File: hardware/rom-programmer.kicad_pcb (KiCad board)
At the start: 2 copper layers, 100 x 68 mm, 21 parts, among them U1 74HC595, U2 74HC595, U3 28C256

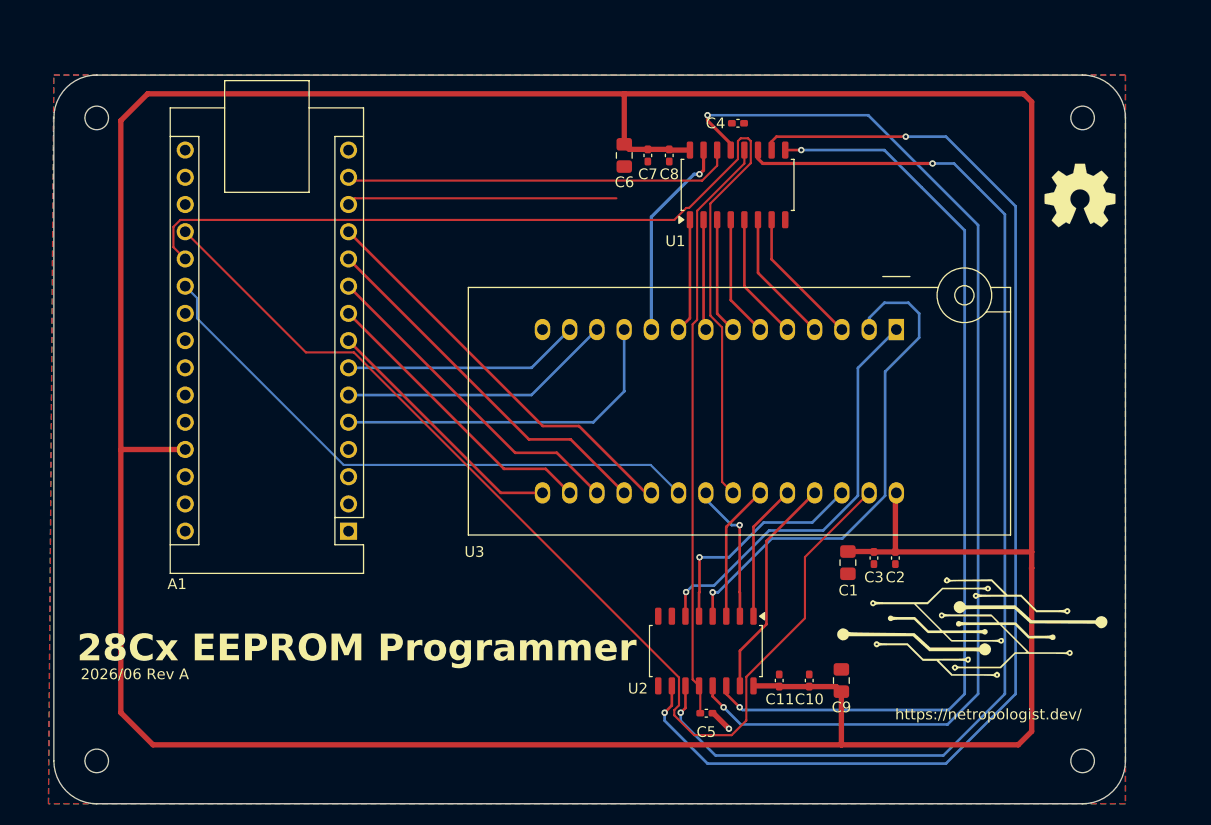
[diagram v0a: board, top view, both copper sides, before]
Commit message: Writing files works
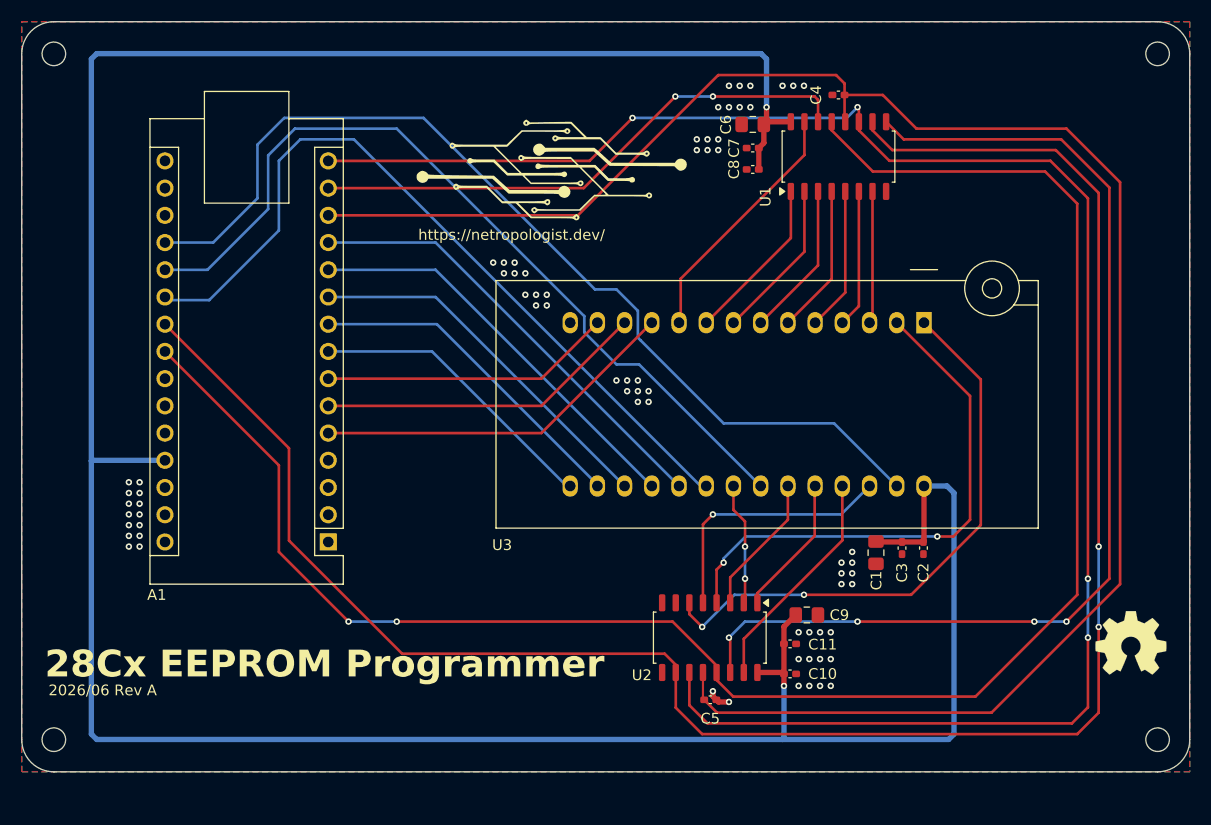
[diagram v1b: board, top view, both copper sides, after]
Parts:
- moved G*** 58.0 mm to (136.5, 71.3)
- moved REF** 42.0 mm to (190.5, 115.5)
- moved C6 12.3 mm to (155.2, 67.1), turned to 180 degrees
- moved C7 9.81 mm to (155.2, 69.3), turned to 180 degrees
- moved U1 9.78 mm to (163.2, 70.1)
- moved C4 9.75 mm to (163.2, 64.4)
- moved H2 9.21 mm to (193.0, 60.5)
- moved C8 7.90 mm to (155.2, 71.3), turned to 180 degrees
- moved H3 7.27 mm to (193.0, 124.5)
- moved H1 7.19 mm to (90.0, 60.5)
- moved C9 6.91 mm to (160.3, 112.9), turned to 0 degrees
- moved H4 4.46 mm to (90.0, 124.5)
- moved C11 3.56 mm to (158.7, 115.6), turned to 0 degrees
- moved C1 2.78 mm to (166.7, 107.1)
- moved C2 2.78 mm to (171.2, 106.6)
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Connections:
- U1 pad 10: /CRCLR -> /~{SRCLR}
- U1 pad 13: /~{SER_OE} -> /~{SEROE}
- U2 pad 10: /CRCLR -> /~{SRCLR}
- U2 pad 13: /~{SER_OE} -> /~{SEROE}
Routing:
- net /~{SRCLR}: track 0.00 -> 184.0 mm, vias 0 -> 2
- net /~{SEROE}: track 0.00 -> 171.0 mm, vias 0 -> 2
- net /CRCLR: track 112.6 -> 0.00 mm, vias 2 -> 0
- net /~{SER_OE}: track 105.4 -> 0.00 mm, vias 2 -> 0
- net /RCLK: track 80.1 -> 171.2 mm
- net +5V: track 340.4 -> 276.7 mm, vias 0 -> 2
- net /SRCLK: track 108.2 -> 166.8 mm, vias 2 -> 4
- net /~{ROM_CE}: track 55.1 -> 74.0 mm
- net /~{ROM_OE}: track 97.1 -> 78.7 mm
- net /SRDATA: track 36.6 -> 51.4 mm, vias 0 -> 2
- net /A14: track 39.0 -> 53.8 mm, vias 1 -> 2
- net /SERO: track 87.3 -> 101.0 mm, vias 2 -> 4
- net /~{ROM_WE}: track 101.1 -> 91.7 mm
- net /D2: track 22.1 -> 27.3 mm
- net /D1: track 25.7 -> 30.9 mm
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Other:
- board size 100 x 68 mm -> 109 x 70 mm
